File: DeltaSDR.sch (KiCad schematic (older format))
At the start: 48 parts, among them J1 Conn_01x03_Male, J2 Conn_01x05_Male, J3 Barrel_Jack, J4 USB_A, U1 TC1262-33, U2 Si570, U4 PCM3060, U5 CY8C3246PVI-147, U6 TLV761, U7 TLV761, U8 74HC74, Y1 Crystal

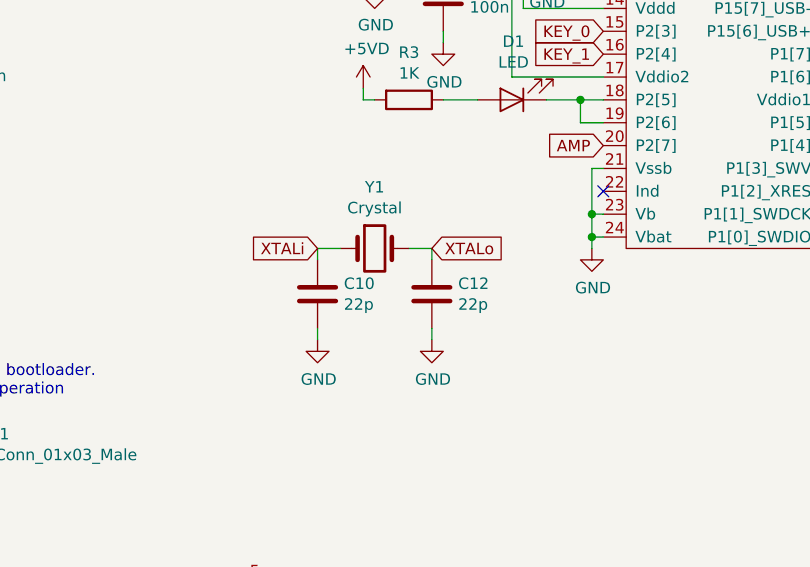
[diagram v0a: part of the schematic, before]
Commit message: First layouting
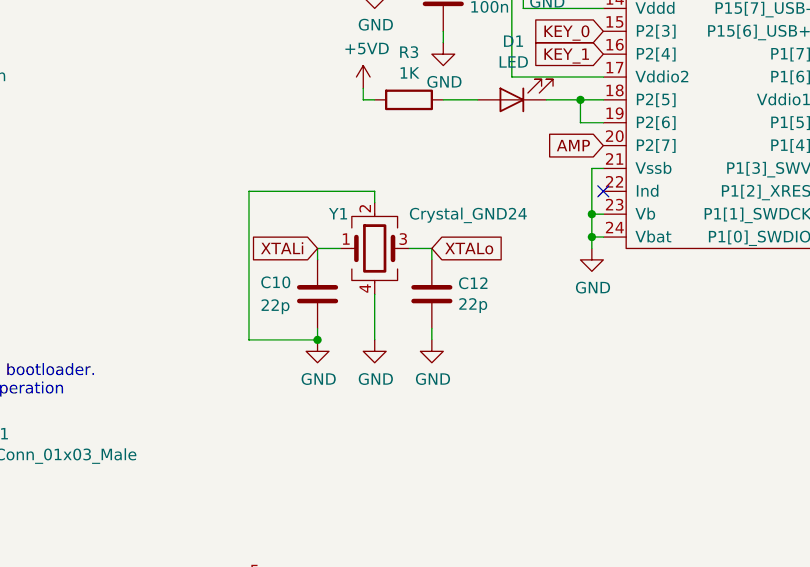
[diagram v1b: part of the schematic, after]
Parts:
- removed Y1: Crystal, symbol DeltaSDR-rescue:Crystal-Device-DeltaSDR-rescue
- added Y1: Crystal_GND24, Crystal:Crystal_SMD_3225-4Pin_3.2x2.5mm, symbol Device:Crystal_GND24
- D1: footprint (none) -> LED_SMD:LED_0805_2012Metric
- D2: footprint (none) -> Diode_SMD:D_SMC
- D3: footprint (none) -> Package_TO_SOT_SMD:SOT-143
- J1: footprint (none) -> Connector_PinHeader_2.54mm:PinHeader_1x03_P2.54mm_Vertical
- J2: footprint (none) -> Connector_PinHeader_2.54mm:PinHeader_1x05_P2.54mm_Vertical
- J3: footprint (none) -> Connector_BarrelJack:BarrelJack_Horizontal
- J4: footprint (none) -> Connector_USB:USB_B_TE_5787834_Vertical
- L1: footprint (none) -> Inductor_SMD:L_0805_2012Metric
- U8: footprint (none) -> Package_SO:SOIC-14_3.9x8.7mm_P1.27mm
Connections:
- net GND: now also Y1.2, Y1.4
- net XTALi: now also Y1.1
- net XTALo: now also Y1.3
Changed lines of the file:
@@
 F 0 "D1" H 7143 4295 50  0000 C CNN
 F 1 "LED" H 7143 4386 50  0000 C CNN
-F 2 "" H 7150 4550 50  0001 C CNN
+F 2 "LED_SMD:LED_0805_2012Metric" H 7150 4550 50  0001 C CNN
 F 3 "~" H 7150 4550 50  0001 C CNN
 	1    7150 4550
@@
 F 0 "J1" V 4762 5762 50  0000 R CNN
 F 1 "Conn_01x03_Male" V 4853 5762 50  0000 R CNN
-F 2 "" H 4700 5950 50  0001 C CNN
+F 2 "Connector_PinHeader_2.54mm:PinHeader_1x03_P2.54mm_Vertical" H 4700 5950 50  0001 C CNN
 F 3 "~" H 4700 5950 50  0001 C CNN
 	1    4700 5950
@@
 BOOT jumper \n1-2 enables USB bootloader.\n2-3 for normal operation
 $Comp
-L DeltaSDR-rescue:Crystal-Device-DeltaSDR-rescue Y1
-U 1 1 5E94EC07
-P 6550 5200
-F 0 "Y1" H 6550 5468 50  0000 C CNN
-F 1 "Crystal" H 6550 5377 50  0000 C CNN
-F 2 "" H 6550 5200 50  0001 C CNN
-F 3 "~" H 6550 5200 50  0001 C CNN
-	1    6550 5200
-	1    0    0    -1
-$EndComp
-$Comp
 L DeltaSDR-rescue:C-Device-DeltaSDR-rescue C10
 U 1 1 5E94F97D
 P 6300 5400
-F 0 "C10" H 6415 5446 50  0000 L CNN
-F 1 "22p" H 6415 5355 50  0000 L CNN
+F 0 "C10" H 6050 5450 50  0000 L CNN
+F 1 "22p" H 6050 5350 50  0000 L CNN
 F 2 "Capacitor_SMD:C_0603_1608Metric" H 6338 5250 50  0001 C CNN
 F 3 "~" H 6300 5400 50  0001 C CNN
@@
 F 0 "J2" H 6122 6782 50  0000 R CNN
 F 1 "Conn_01x05_Male" H 6122 6873 50  0000 R CNN
-F 2 "" H 6150 6850 50  0001 C CNN
+F 2 "Connector_PinHeader_2.54mm:PinHeader_1x05_P2.54mm_Vertical" H 6150 6850 50  0001 C CNN
 F 3 "~" H 6150 6850 50  0001 C CNN
 	1    6150 6850
@@
 F 0 "J3" H 1154 1375 50  0000 C CNN
 F 1 "Barrel_Jack" H 1154 1284 50  0000 C CNN
-F 2 "" H 1125 1010 50  0001 C CNN
+F 2 "Connector_BarrelJack:BarrelJack_Horizontal" H 1125 1010 50  0001 C CNN
 F 3 "~" H 1125 1010 50  0001 C CNN
 	1    1075 1050
@@
 F 0 "D2" H 1650 734 50  0000 C CNN
 F 1 "D" H 1650 825 50  0000 C CNN
-F 2 "" H 1650 950 50  0001 C CNN
+F 2 "Diode_SMD:D_SMC" H 1650 950 50  0001 C CNN
 F 3 "" H 1650 950 50  0001 C CNN
 	1    1650 950
@@
 F 0 "L1" V 2240 950 50  0000 C CNN
 F 1 "74279220321" V 2149 950 50  0000 C CNN
-F 2 "" H 2050 950 50  0001 C CNN
+F 2 "Inductor_SMD:L_0805_2012Metric" H 2050 950 50  0001 C CNN
 F 3 "" H 2050 950 50  0001 C CNN
 	1    2050 950
@@
 F 0 "U8" H 3000 2975 50  0000 C CNN
 F 1 "74HC74" H 3325 2475 50  0000 C CNN
-F 2 "" H 3150 2725 50  0001 C CNN
+F 2 "Package_SO:SOIC-14_3.9x8.7mm_P1.27mm" H 3150 2725 50  0001 C CNN
 F 3 "74xx/74hc_hct74.pdf" H 3150 2725 50  0001 C CNN
 	1    3150 2725
@@
 F 0 "U8" H 3875 2975 50  0000 C CNN
 F 1 "74HC74" H 4200 2475 50  0000 C CNN
-F 2 "" H 4025 2725 50  0001 C CNN
+F 2 "Package_SO:SOIC-14_3.9x8.7mm_P1.27mm" H 4025 2725 50  0001 C CNN
 F 3 "74xx/74hc_hct74.pdf" H 4025 2725 50  0001 C CNN
 	2    4025 2725
@@
 F 0 "U8" H 4800 2975 50  0000 L CNN
 F 1 "74HC74" H 5075 2250 50  0000 L CNN
-F 2 "" H 5025 2625 50  0001 C CNN
+F 2 "Package_SO:SOIC-14_3.9x8.7mm_P1.27mm" H 5025 2625 50  0001 C CNN
 F 3 "74xx/74hc_hct74.pdf" H 5025 2625 50  0001 C CNN
 	3    5025 2625
@@
 F 0 "J4" H 2157 7142 50  0000 C CNN
 F 1 "USB_A" H 2157 7051 50  0000 C CNN
-F 2 "" H 2250 6625 50  0001 C CNN
+F 2 "Connector_USB:USB_B_TE_5787834_Vertical" H 2250 6625 50  0001 C CNN
 F 3 "" H 2250 6625 50  0001 C CNN
 	1    2100 6675
@@
 F 0 "D3" H 2925 6442 50  0000 C CNN
 F 1 "PRTR5V0U2X" H 2925 6351 50  0000 C CNN
-F 2 "" H 2975 6025 50  0001 C CNN
+F 2 "Package_TO_SOT_SMD:SOT-143" H 2975 6025 50  0001 C CNN
 F 3 "https://assets.nexperia.com/documents/data-sheet/PRTR5V0U2X.pdf" H 2975 6025 50  0001 C CNN
 	1    2925 6075
@@
 Wire Wire Line
 	2400 950  2550 950
+$Comp
+L Device:Crystal_GND24 Y1
+U 1 1 5E9781A4
+P 6550 5200
+F 0 "Y1" H 6350 5350 50  0000 L CNN
+F 1 "Crystal_GND24" H 6700 5350 50  0000 L CNN
+F 2 "Crystal:Crystal_SMD_3225-4Pin_3.2x2.5mm" H 6550 5200 50  0001 C CNN
+F 3 "~" H 6550 5200 50  0001 C CNN
+	1    6550 5200
+	1    0    0    -1
+$EndComp
+$Comp
+L power:GND #PWR0221
+U 1 1 5E9783E9
+P 6550 5600
+F 0 "#PWR0221" H 6550 5350 50  0001 C CNN
+F 1 "GND" H 6555 5427 50  0000 C CNN
+F 2 "" H 6550 5600 50  0001 C CNN
+F 3 "" H 6550 5600 50  0001 C CNN
+	1    6550 5600
+	1    0    0    -1
+$EndComp
+Wire Wire Line
+	6550 5400 6550 5600
+Wire Wire Line
+	6550 5000 6550 4950
+Wire Wire Line
+	6550 4950 6000 4950
+Wire Wire Line
+	6000 4950 6000 5600
+Wire Wire Line
+	6000 5600 6300 5600
+Connection ~ 6300 5600
 $EndSCHEMATC
